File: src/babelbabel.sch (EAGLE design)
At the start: 86 parts, among them CON1 CON-4P-TABS-JST_GH-RA, CON10 CON-6P-SM06B, CON11 PINHEAD_1X04-2.54, CON12 PINHEAD_1X06-2.54, CON15 PINHEAD_1X04-2.54, CON16 CON-4P-TABS-JST_GH-RA, CON2 PINHEAD_1X04-2.54, CON3 PINHEAD_1X04-2.54, CON4 USB-AA-PTH, CON5 CON-4P-TABS-JST_GH-RA, CON6 CON-4P-TABS-JST_GH-RA, CON7 USB-1, IC1 NS5B1G385, IC13 STM32F103CBT7, IC14 74LVC2T45, IC15 74LVC2T45, IC16 74LVC2T45, IC17 74LVC2T45, IC2 NS5B1G385, IC3 AP2127-3.3, IC9 FE1.1S, J1 CONNECTION-SMD, J2 CONNECTION-SMD, Q7 8MHz, Q8 12MHz, Q9 NTZD3152PT1G

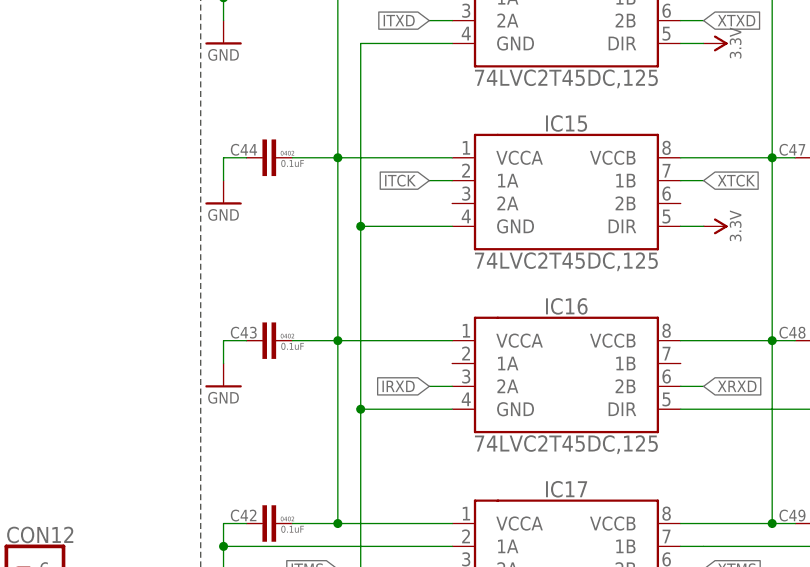
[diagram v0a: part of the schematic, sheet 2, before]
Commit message: Revert "source files consistency fix"
This reverts commit 015ba0159d9c48fa3345c98b8ff1ca9c9c6bfb7d.
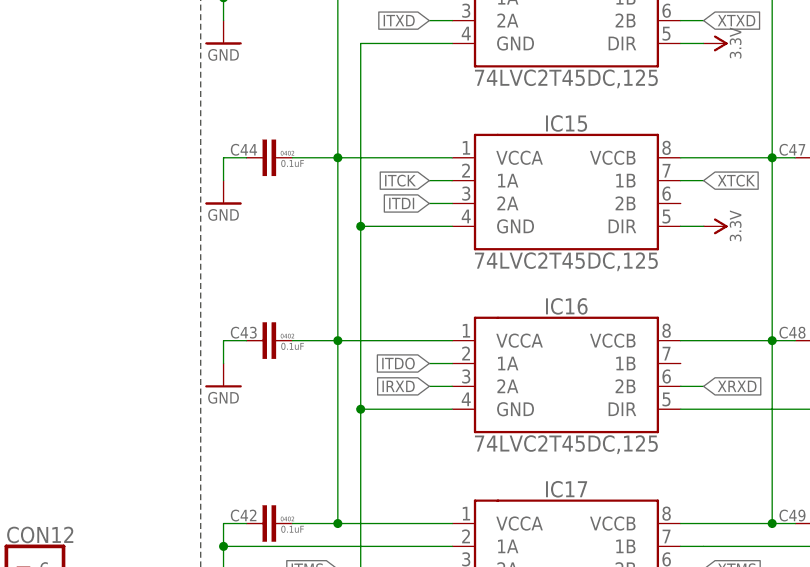
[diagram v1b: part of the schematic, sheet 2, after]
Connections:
- new net ITDI: IC15.2A
- new net ITDO: IC16.1A
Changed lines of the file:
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@@
 </ports>
 <variantdefs>
-<variantdef name="48_pin_MCU"/>
-<variantdef name="64_pin_MCU"/>
+<variantdef name="A"/>
+<variantdef name="basic"/>
 </variantdefs>
 <parts>
 <part name="IC1" library="stm32" library_urn="urn:adsk.eagle:library:2473361" deviceset="STM32F373CBT6" device="-LQFP48" package3d_urn="urn:adsk.eagle:package:2473350/4">
-<variant name="64_pin_MCU" populate="no"/>
+<variant name="basic" populate="no"/>
 </part>
 <part name="GND1" library="supply_symbols" library_urn="urn:adsk.eagle:library:5017758" deviceset="GND" device="" value="GND"/>
@@
 <part name="P+6" library="supply_symbols" library_urn="urn:adsk.eagle:library:5017758" deviceset="3.3V" device=""/>
 <part name="GND4" library="supply_symbols" library_urn="urn:adsk.eagle:library:5017758" deviceset="GND" device="" value="GND"/>
-<part name="IC8" library="misc" library_urn="urn:adsk.eagle:library:5347860" deviceset="TPD3S014DBVR" device="-SOT23-6" package3d_urn="urn:adsk.eagle:package:1040217/3"/>
+<part name="IC8" library="misc" library_urn="urn:adsk.eagle:library:5347860" deviceset="TPD3S014DBVR" device="-SOT23-6" package3d_urn="urn:adsk.eagle:package:1040217/3">
+<variant name="A" populate="no"/>
+</part>
 <part name="+P4" library="supply_symbols" library_urn="urn:adsk.eagle:library:13097679" deviceset="5V" device=""/>
 <part name="C84" library="rc" library_urn="urn:adsk.eagle:library:2539423" deviceset="C" device="-0402" package3d_urn="urn:adsk.eagle:package:2539461/2" value="0.1uF">
@@
 <part name="IC2" library="stm32" library_urn="urn:adsk.eagle:library:2473361" deviceset="STM32F373RCT6" device="" package3d_urn="urn:adsk.eagle:package:2473349/4">
 <attribute name="DIGIKEY#" value="497-13252-ND"/>
-<variant name="48_pin_MCU" populate="no"/>
 </part>
 <part name="P+11" library="supply_symbols" library_urn="urn:adsk.eagle:library:5017758" deviceset="3.3V" device=""/>
@@
 <pinref part="IC1" gate="G$1" pin="BOOT0"/>
 <pinref part="R11" gate="G$1" pin="2"/>
-<label x="265.684" y="164.084" size="1.27" layer="95" rot="R90"/>
 </segment>
 <segment>
@@
 <part name="+P40" library="supply_symbols" library_urn="urn:adsk.eagle:library:5017758" deviceset="3.3V" device=""/>
 <part name="GND90" library="supply_symbols" library_urn="urn:adsk.eagle:library:5017758" deviceset="GND" device="" value="GND"/>
-<part name="CON11" library="pinhead" library_urn="urn:adsk.eagle:library:2540341" deviceset="PINHEAD_1X04" device="-2.54" package3d_urn="urn:adsk.eagle:package:2540383/2">
-<variant name="Electronic terminator" populate="no"/>
-<variant name="Mechanical terminator" populate="no"/>
-</part>
+<part name="CON11" library="pinhead" library_urn="urn:adsk.eagle:library:2540341" deviceset="PINHEAD_1X04" device="-2.54" package3d_urn="urn:adsk.eagle:package:2540383/2"/>
 <part name="CON12" library="pinhead" library_urn="urn:adsk.eagle:library:2540341" deviceset="PINHEAD_1X06" device="-2.54" package3d_urn="urn:adsk.eagle:package:2540381/2"/>
 <part name="GND91" library="supply_symbols" library_urn="urn:adsk.eagle:library:5017758" deviceset="GND" device="" value="GND"/>
@@
 </plain>
 <moduleinsts>
-<moduleinst name="BABEL1" module="BABEL" modulevariant="64_pin_MCU" x="190.5" y="134.62" offset="100">
+<moduleinst name="BABEL1" module="BABEL" modulevariant="basic" x="190.5" y="134.62" offset="100">
 <attribute name="NAME" x="190.5" y="145.796" size="2.032" layer="95" align="bottom-center"/>
 </moduleinst>
-<moduleinst name="BABEL2" module="BABEL" modulevariant="64_pin_MCU" x="190.5" y="60.96" offset="200">
+<moduleinst name="BABEL2" module="BABEL" modulevariant="basic" x="190.5" y="60.96" offset="200">
 <attribute name="NAME" x="190.5" y="72.136" size="2.032" layer="95" align="bottom-center"/>
 </moduleinst>
@@
 </segment>
 </net>
+<net name="ITDI" class="0">
+<segment>
+<pinref part="IC15" gate="G$1" pin="2A"/>
+<wire x1="203.2" y1="137.16" x2="200.66" y2="137.16" width="0.1524" layer="91"/>
+<label x="200.66" y="137.16" size="1.27" layer="95" rot="R180" xref="yes"/>
+</segment>
+</net>
 <net name="XTCK" class="0">
 <segment>
@@
 </segment>
 </net>
+<net name="ITDO" class="0">
+<segment>
+<pinref part="IC16" gate="G$1" pin="1A"/>
+<wire x1="203.2" y1="119.38" x2="200.66" y2="119.38" width="0.1524" layer="91"/>
+<label x="200.66" y="119.38" size="1.27" layer="95" rot="R180" xref="yes"/>
+</segment>
+</net>
